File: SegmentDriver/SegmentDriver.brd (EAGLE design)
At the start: 175 x 175 mm, 221 parts, among them IC1 ATMEGA644A, IC2 PCA9555PW, IC3 4511D, K1 691313710002, K10 M02-MOLEX-104188-0210, K11 M02-MOLEX-104188-0210, K12 M02-MOLEX-104188-0210, K13 M02-MOLEX-104188-0210, K14 M02-MOLEX-104188-0210, K15 M02-MOLEX-104188-0210, K16 M02-MOLEX-104188-0210, K17 691210910004, K18 691210910004, K19 691210910004, K2 691313710002, K20 691210910004, K21 691210910004, K22 691210910004, K23 691210910004, K24 691210910004, K25 691210910004, K3 691322310002, K4 691322310002, K6 61200621621, K7 61201021621, K8 M02-MOLEX-104188-0210, K9 M02-MOLEX-104188-0210, Q1 MOSFET-NCHANNEL-FDMS5672, Q2 MOSFET-NCHANNEL-FDMS5672, Q3 MOSFET-NCHANNEL-FDMS5672, Q4 MOSFET-NCHANNEL-FDMS5672, Q5 MOSFET-NCHANNEL-FDMS5672, Q6 MOSFET-NCHANNEL-FDMS5672, Q7 MOSFET-NCHANNEL-FDMS5672, Q8 MOSFET-NCHANNEL-FDMS5672, Q9 MOSFET-NCHANNEL-FDMS5672, SW1 SPST_TACT-EVQQ2, U1 DS1307SO8-TIGHT, U10 FOD8321, U11 FOD8321, U15 DMP2215L-7, U16 DMP2215L-7, U3 FOD8321, U4 FOD8321, U5 FOD8321, U6 FOD8321, U7 FOD8321, U8 FOD8321, U9 FOD8321, X1 53261-03, X2 53261-03, X3 53261-03, X4 53261-03, X5 53261-03, X6 53261-03, Y2 32.768kHz

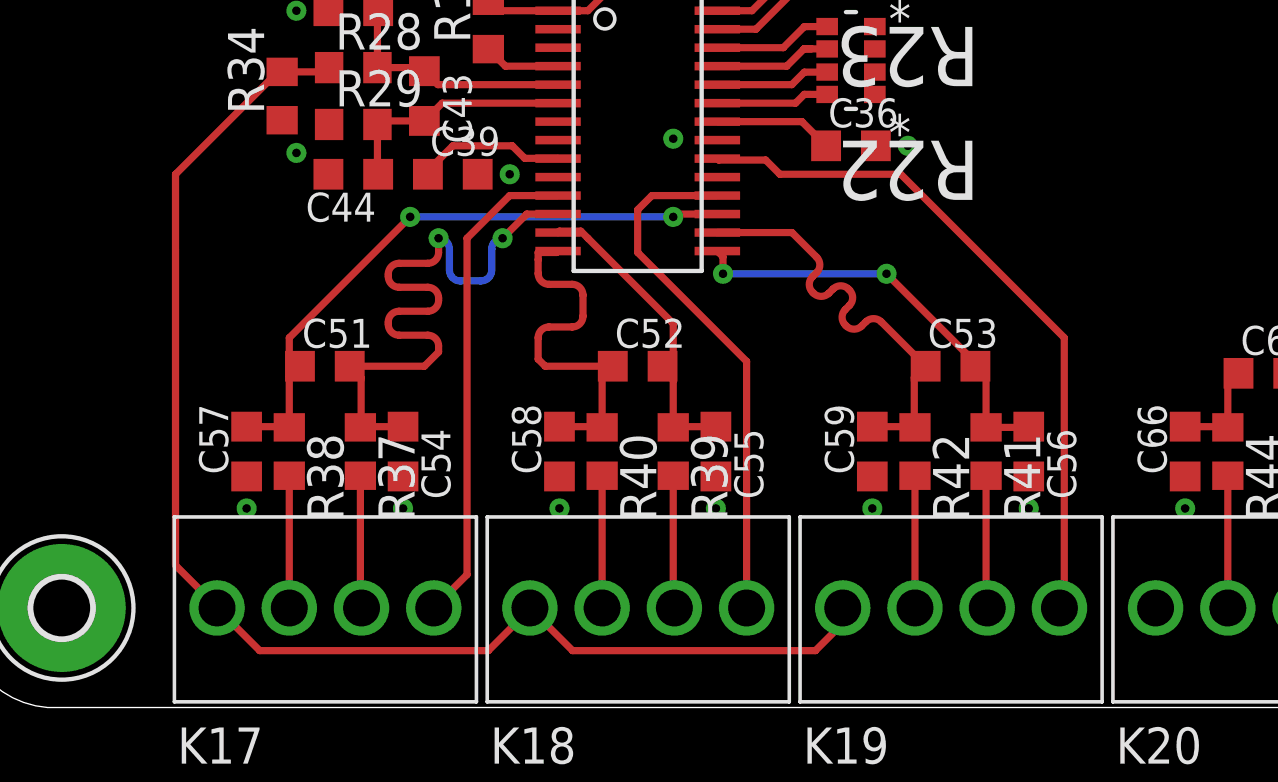
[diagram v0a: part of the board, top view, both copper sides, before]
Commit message: small repositioning
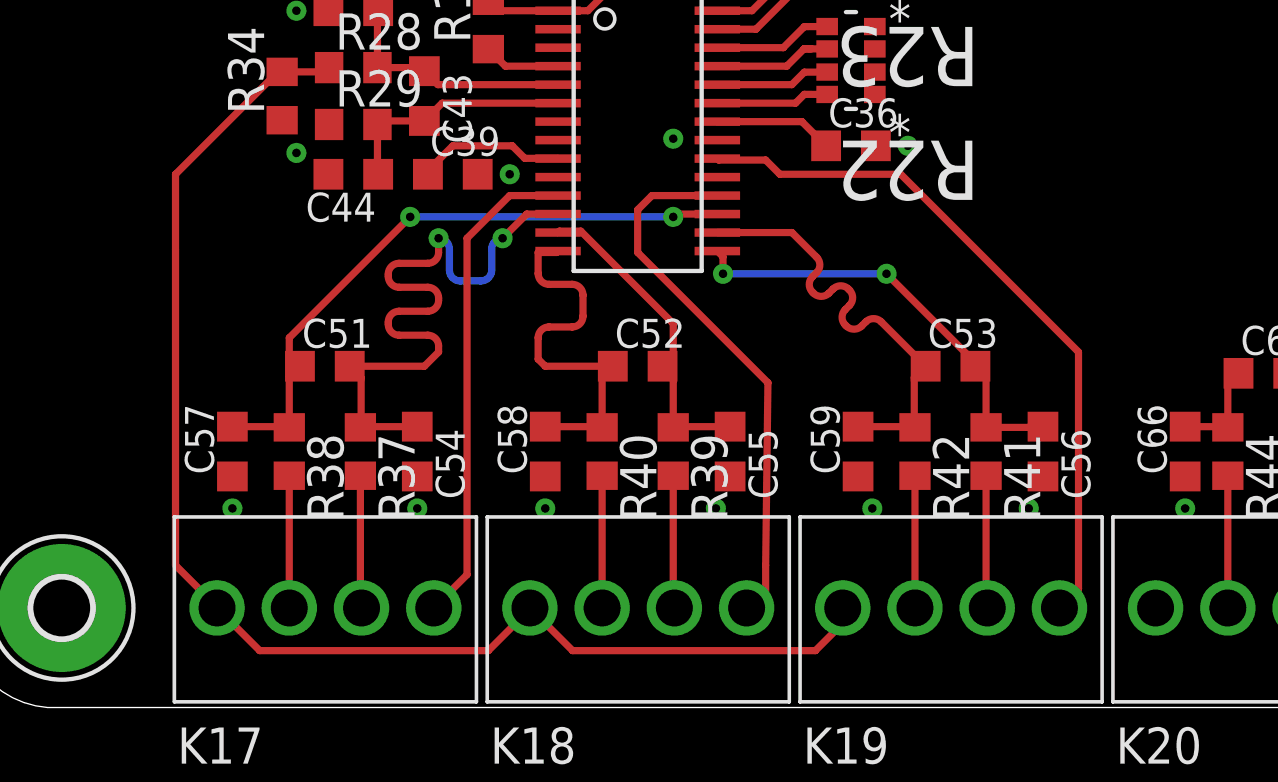
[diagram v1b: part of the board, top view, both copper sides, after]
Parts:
- moved C54 0.50 mm to (16.0, 9.00)
- moved C55 0.50 mm to (27.0, 9.00)
- moved C56 0.50 mm to (38.0, 9.00)
- moved C57 0.50 mm to (9.50, 9.00)
- moved C58 0.50 mm to (20.5, 9.00)
- moved C59 0.50 mm to (31.5, 9.00)
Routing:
- net AD1_AIN3: track 18.6 -> 19.6 mm
- net AD1_AIN1: track 23.5 -> 24.0 mm
- net AD1_AIN5: track 13.3 -> 13.8 mm
- net AD1_AIN7: track 15.2 -> 15.7 mm
- net AD1_AIN2: track 22.0 -> 22.5 mm
